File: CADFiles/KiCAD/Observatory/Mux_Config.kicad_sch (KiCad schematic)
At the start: 18 parts, among them J17 WaveGen. 1 Mux Config., J4 Scope 1 Mux Config., J5 Scope 2 Mux Config.

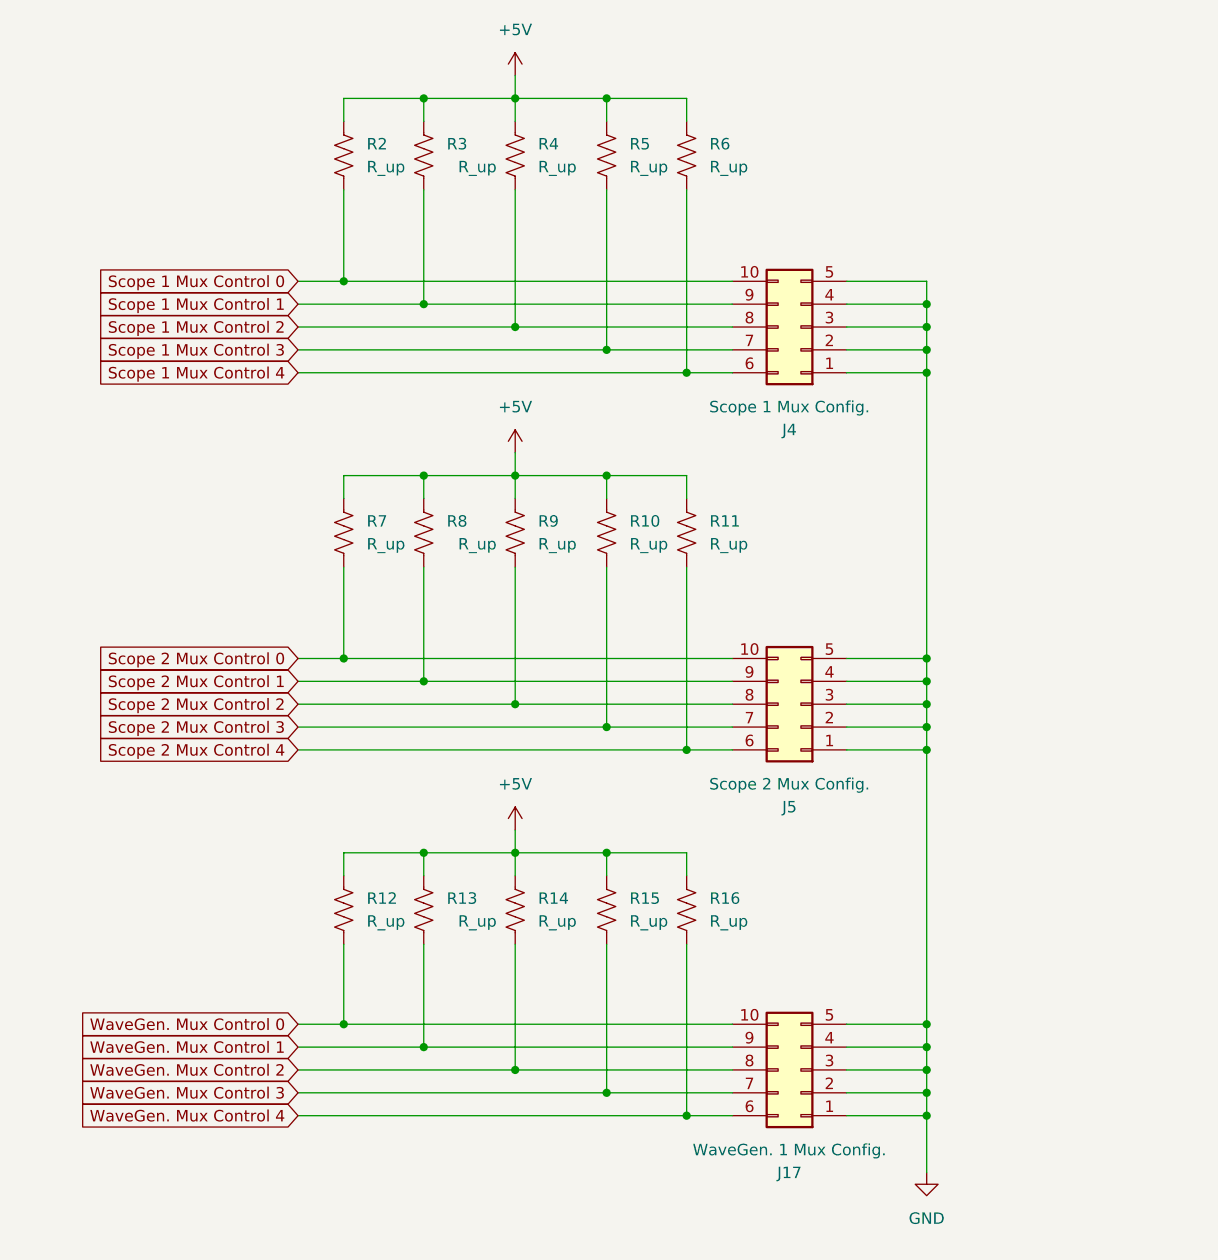
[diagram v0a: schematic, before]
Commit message: Begin REV 2
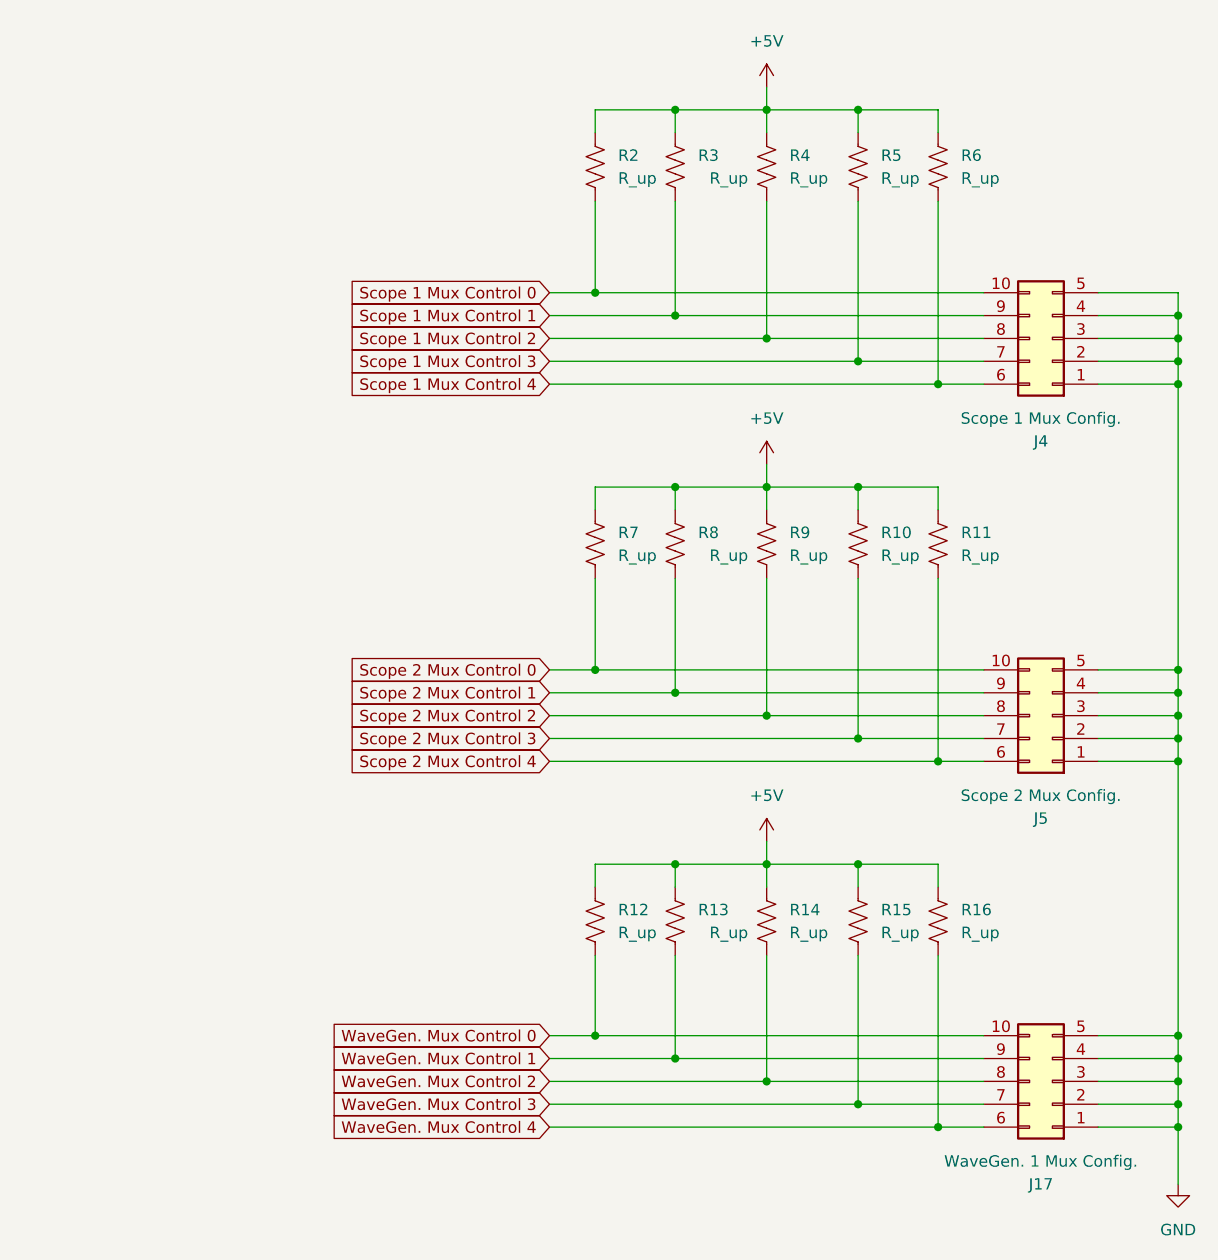
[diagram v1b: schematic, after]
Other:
- moved on the sheet: J17, J4, J5, R10, R11, R12, R13, R14, R15, R16, R2, R3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

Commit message: All nets routed.
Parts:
- J17, J4, J5: footprint Imports:DIP8_208-5_CTS -> Button_Switch_SMD:SW_DIP_SPSTx05_Slide_6.7x14.26mm_W8.61mm_P2.54mm_LowProfile
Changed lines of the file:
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@@
 			)
 		)
-		(property "Footprint" "Imports:DIP8_208-5_CTS"
+		(property "Footprint" "Button_Switch_SMD:SW_DIP_SPSTx05_Slide_6.7x14.26mm_W8.61mm_P2.54mm_LowProfile"
 			(at 162.56 100.33 0)
 			(effects
@@
 			)
 		)
-		(property "Footprint" "Imports:DIP8_208-5_CTS"
+		(property "Footprint" "Button_Switch_SMD:SW_DIP_SPSTx05_Slide_6.7x14.26mm_W8.61mm_P2.54mm_LowProfile"
 			(at 162.56 58.42 0)
 			(effects
@@
 			)
 		)
-		(property "Footprint" "Imports:DIP8_208-5_CTS"
+		(property "Footprint" "Button_Switch_SMD:SW_DIP_SPSTx05_Slide_6.7x14.26mm_W8.61mm_P2.54mm_LowProfile"
 			(at 162.56 140.97 0)
 			(effects

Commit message: AD DC(-) error fixed. Jumpers added for feet grounds and DC supplies
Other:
- company: (none) -> West Lab
- title: (none) -> SCuM Observatory
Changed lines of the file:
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@@
 	(generator_version "9.0")
 	(paper "A4")
+	(title_block
+		(title "SCuM Observatory")
+		(date "2025-03-21")
+		(rev "2")
+		(company "West Lab")
+	)
 	(junction
 		(at 176.53 60.96)
